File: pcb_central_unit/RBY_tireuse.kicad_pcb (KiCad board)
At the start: 2 copper layers, 120.6 x 80 mm, 10 parts, among them J1 CMD_PAN, J2 GLASS_0, J3 GLASS_1, J4 Conn_01x04_Female, J5 Conn_01x04_Female, J6 DCDC_BOOSTER, J7 Conn_01x02_Male, U1 ESP32-DEVKITC-32D, U2 TMC2208_SILENTSTEPSTICK, U3 TMC2208_SILENTSTEPSTICK

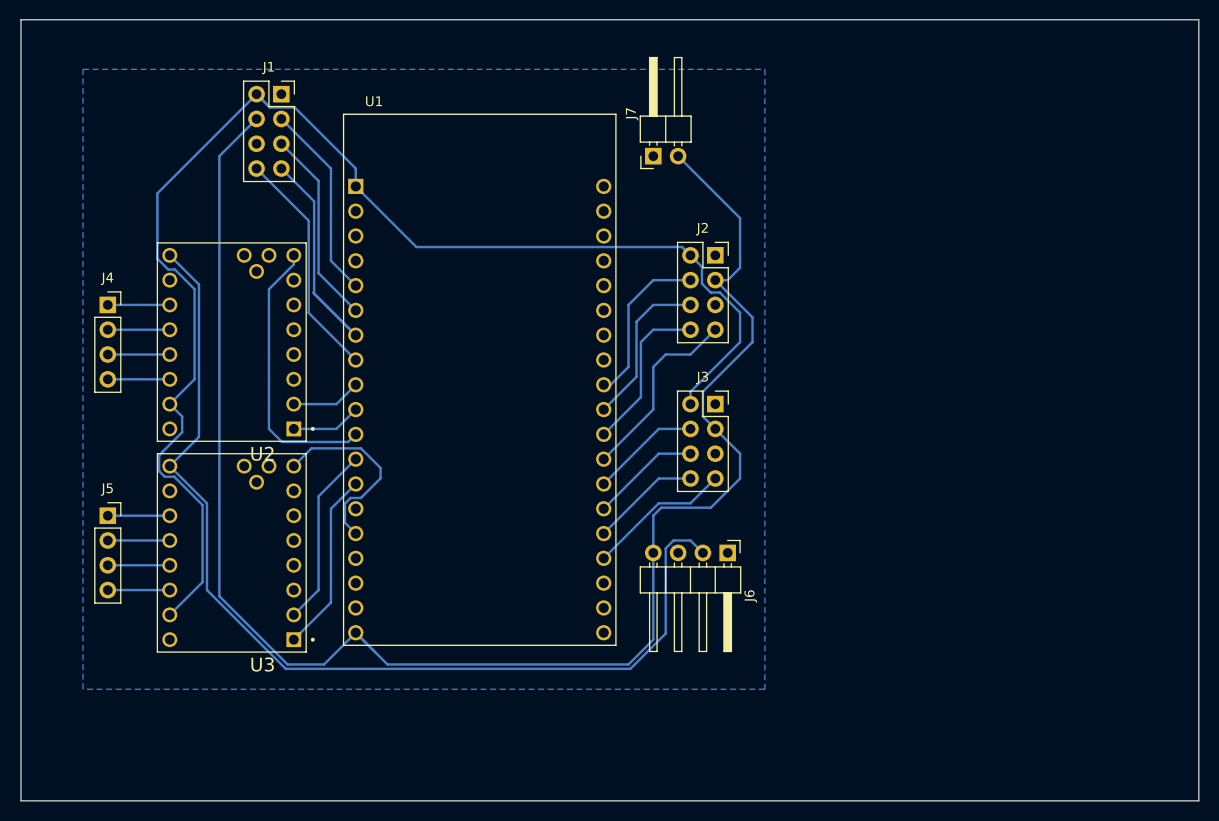
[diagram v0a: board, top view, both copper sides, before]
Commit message: PCB V2
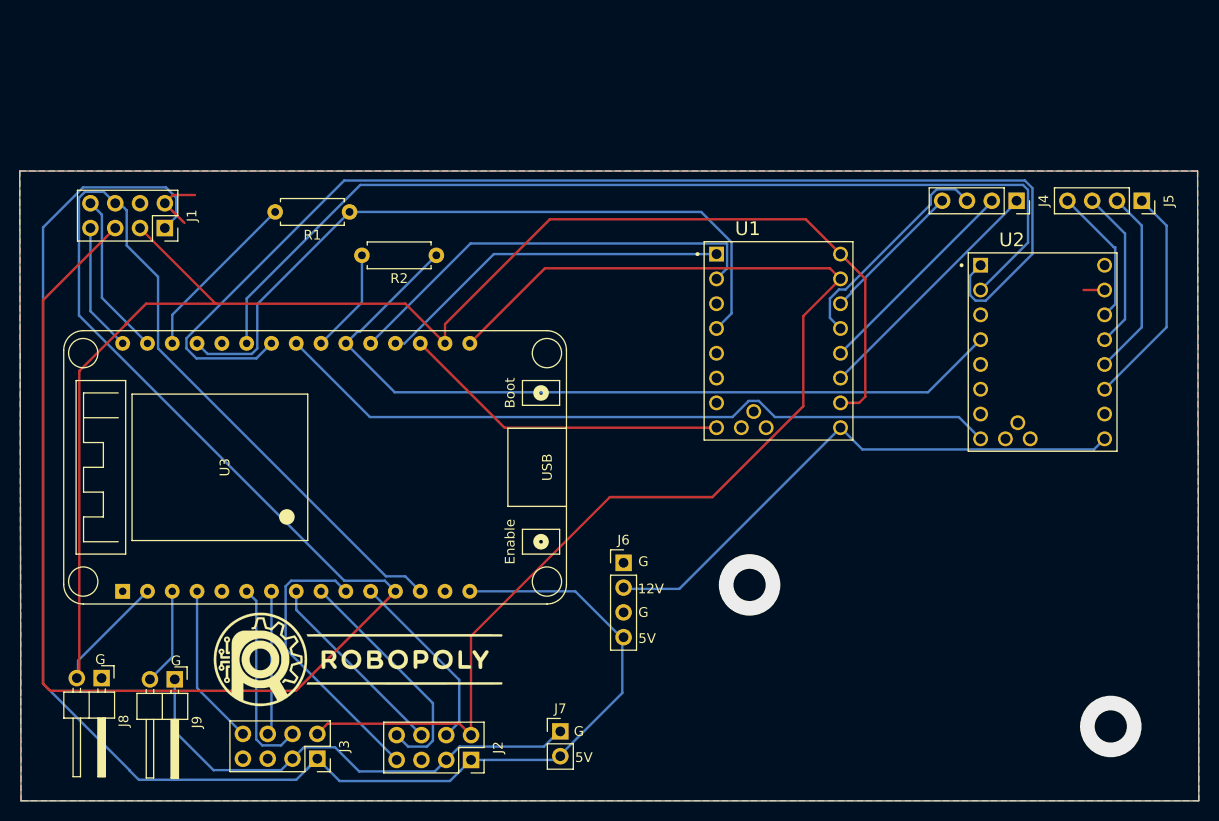
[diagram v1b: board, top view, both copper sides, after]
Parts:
- added J8: SPARE_GPIO_0, Connector_PinHeader_2.54mm:PinHeader_1x02_P2.54mm_Horizontal, F.Cu at (55.2, 114.4)
- added J9: SPARE_GPIO_1, Connector_PinHeader_2.54mm:PinHeader_1x02_P2.54mm_Horizontal, F.Cu at (62.7, 114.6)
- added R1: 1kOHM, Resistor_THT:R_Axial_DIN0207_L6.3mm_D2.5mm_P7.62mm_Horizontal, F.Cu at (80.6, 66.7)
- added R2: 1kOHM, Resistor_THT:R_Axial_DIN0207_L6.3mm_D2.5mm_P7.62mm_Horizontal, F.Cu at (89.5, 71.1)
- added REF**: logo_30mm, robopoly_logo:logo_30mm, F.Cu at (83.7, 112.4)
- added REF**: logo_50mm, robopoly_logo:logo_50mm, B.Cu at (83.1, 95.0)
- J4: value Conn_01x04_Female -> STEPPER_0
- J5: value Conn_01x04_Female -> STEPPER_1
- J6: footprint Connector_PinHeader_2.54mm:PinHeader_1x04_P2.54mm_Horizontal -> Connector_PinHeader_2.54mm:PinHeader_1x04_P2.54mm_Vertical
- J7: value Conn_01x02_Male -> ALIM_5V; footprint Connector_PinHeader_2.54mm:PinHeader_1x02_P2.54mm_Horizontal -> Connector_PinHeader_2.54mm:PinHeader_1x02_P2.54mm_Vertical
- U1: value ESP32-DEVKITC-32D -> TMC2208_SILENTSTEPSTICK-TMC2208_SILENTSTEPSTICK; footprint MODULE_ESP32:MODULE_ESP32-DEVKITC-32D -> ProjectModules:MODULE_TMC2208_SILENTSTEPSTICK
- U2: value TMC2208_SILENTSTEPSTICK -> TMC2208_SILENTSTEPSTICK-TMC2208_SILENTSTEPSTICK; footprint MODULE_ESP32:MODULE_TMC2208_SILENTSTEPSTICK -> ProjectModules:MODULE_TMC2208_SILENTSTEPSTICK
- U3: value TMC2208_SILENTSTEPSTICK -> ESP32_DevKit_V1_DOIT_30_pin; footprint MODULE_ESP32:MODULE_TMC2208_SILENTSTEPSTICK -> ProjectModules:esp32_devkit_v1_doit
- moved J5 110.7 mm to (161.8, 65.5), turned to 270 degrees
- moved J4 93.7 mm to (149.0, 65.5), turned to 270 degrees
- moved U2 83.1 mm to (151.6, 81.0), turned to 0 degrees
- moved J7 59.7 mm to (102.2, 119.9), turned to 0 degrees
- moved J2 57.4 mm to (93.1, 122.8), turned to 270 degrees
- moved J3 54.6 mm to (77.3, 122.7), turned to 270 degrees
- moved U1 30.9 mm to (124.6, 79.9)
- moved J1 18.2 mm to (61.7, 68.3), turned to 270 degrees
- moved U3 14.2 mm to (57.4, 92.8), turned to 90 degrees
- moved J6 10.7 mm to (108.7, 102.6), turned to 0 degrees
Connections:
- J1 pad 1: GND -> +5V
- J1 pad 3: B1 -> GND
- J1 pad 4: +5V -> Net-(J1-Pad4)
- J1 pad 5: B2 -> B1
- J1 pad 6: Net-(J1-Pad6) -> B2
- J2 pad 1: GND -> +5V
- J2 pad 3: +5V -> GND
- J3 pad 1: GND -> +5V
- J3 pad 3: +5V -> GND
- J6 pad 1: GNDPWR -> GND
- U2 pad JP1_1: DIR_0 -> DIR_1
- U2 pad JP1_2: PULS_0 -> PULS_1
- U2 pad JP1_4: Net-(U2-PadJP1_4) -> UART_1
- U2 pad JP1_8: EN_0 -> EN_1
- U2 pad JP2_3: Net-(J4-Pad1) -> Net-(J5-Pad1)
- U2 pad JP2_4: Net-(J4-Pad2) -> Net-(J5-Pad2)
- U2 pad JP2_5: Net-(J4-Pad3) -> Net-(J5-Pad3)
- U2 pad JP2_6: Net-(J4-Pad4) -> Net-(J5-Pad4)
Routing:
- net GND: track 0.56 -> 201.5 mm
- net B1: track 20.2 -> 151.0 mm
- net DIR_1: track 18.6 -> 123.3 mm
- net PULS_1: track 18.6 -> 101.9 mm
- net UART_1: track 0.00 -> 82.3 mm
- net UART_0: track 0.00 -> 74.6 mm
- net EN_1: track 19.8 -> 75.5 mm
- net +12V: track 103.6 -> 57.6 mm
- net PULS_0: track 7.17 -> 44.8 mm
- net B2: track 20.2 -> 53.7 mm
- net DIR_0: track 7.17 -> 36.7 mm
- net Net-(J4-Pad1): track 6.35 -> 25.6 mm
- net Net-(R1-Pad2): track 0.00 -> 17.8 mm
- net Net-(J4-Pad3): track 6.35 -> 23.2 mm
- net Net-(J5-Pad1): track 6.35 -> 23.0 mm
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- added copper zone on F.Cu, net +3.3V
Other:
- board size 120.6 x 80 mm -> 120.8 x 64.5 mm
- board text added: "12V"
- board text added: "5V"
- board text added: "G"
